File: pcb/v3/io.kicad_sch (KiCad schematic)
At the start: 54 parts, among them J12 Conn_01x04, J13 Conn_01x05, P1 LCD_MIPI, P2 LCD_TOUCH, U10 STI9287, Y1 24.576M

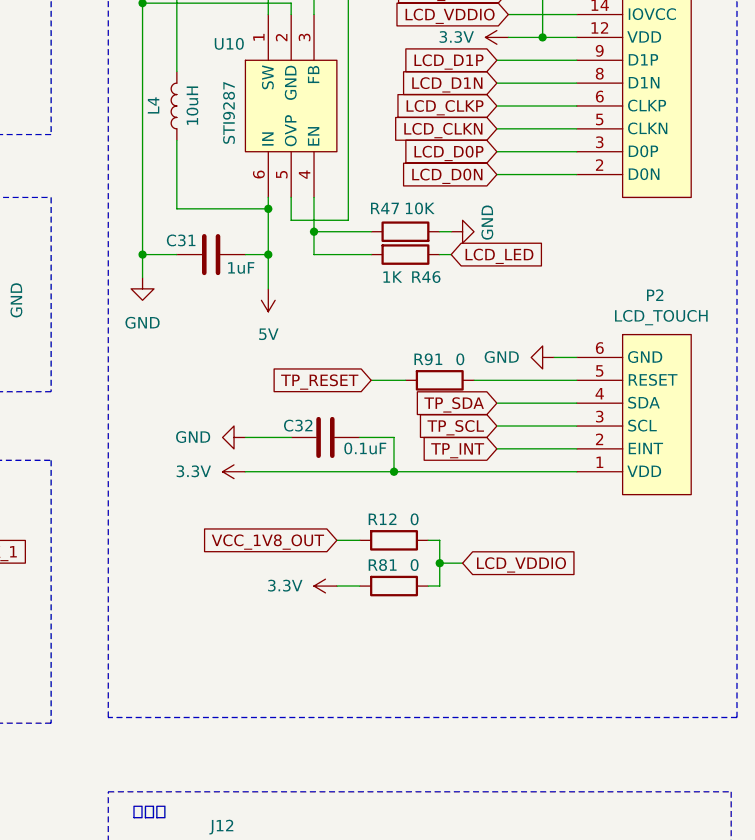
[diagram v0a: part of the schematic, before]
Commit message: up
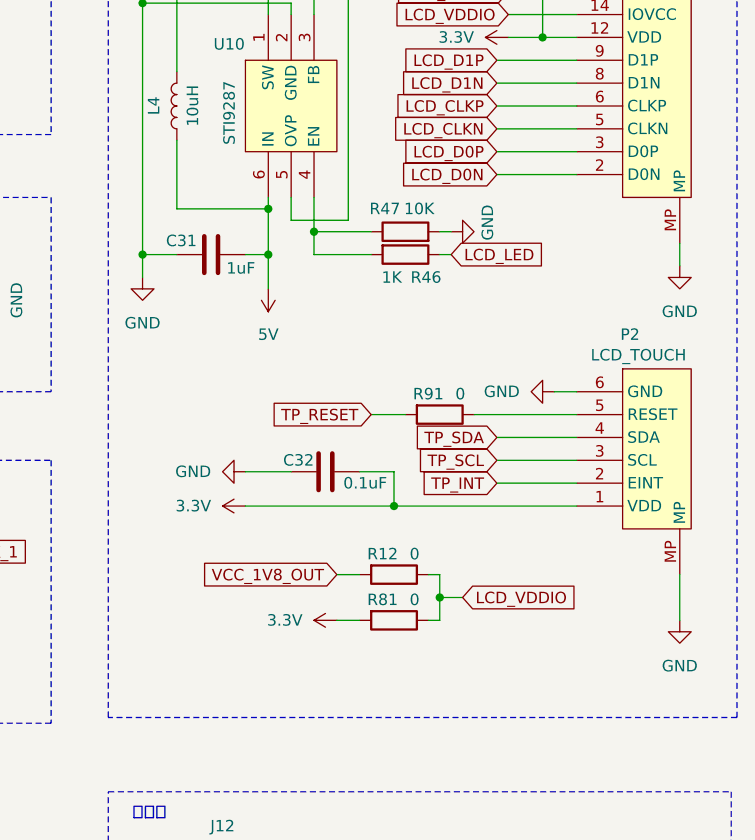
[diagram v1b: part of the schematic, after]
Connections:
- net GND: now also P1.MP, P2.MP
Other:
- moved on the sheet: C32, R12, R81, R91
